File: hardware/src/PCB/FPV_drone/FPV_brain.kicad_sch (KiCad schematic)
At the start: 35 parts, among them IC2 STM32H743VIT6, IC3 USBLC6-2SC6, J1 TYPE-C-31-M-12, J3 Flash-pads, Y1 ABM3B-8.000MHZ-10-D1G-T

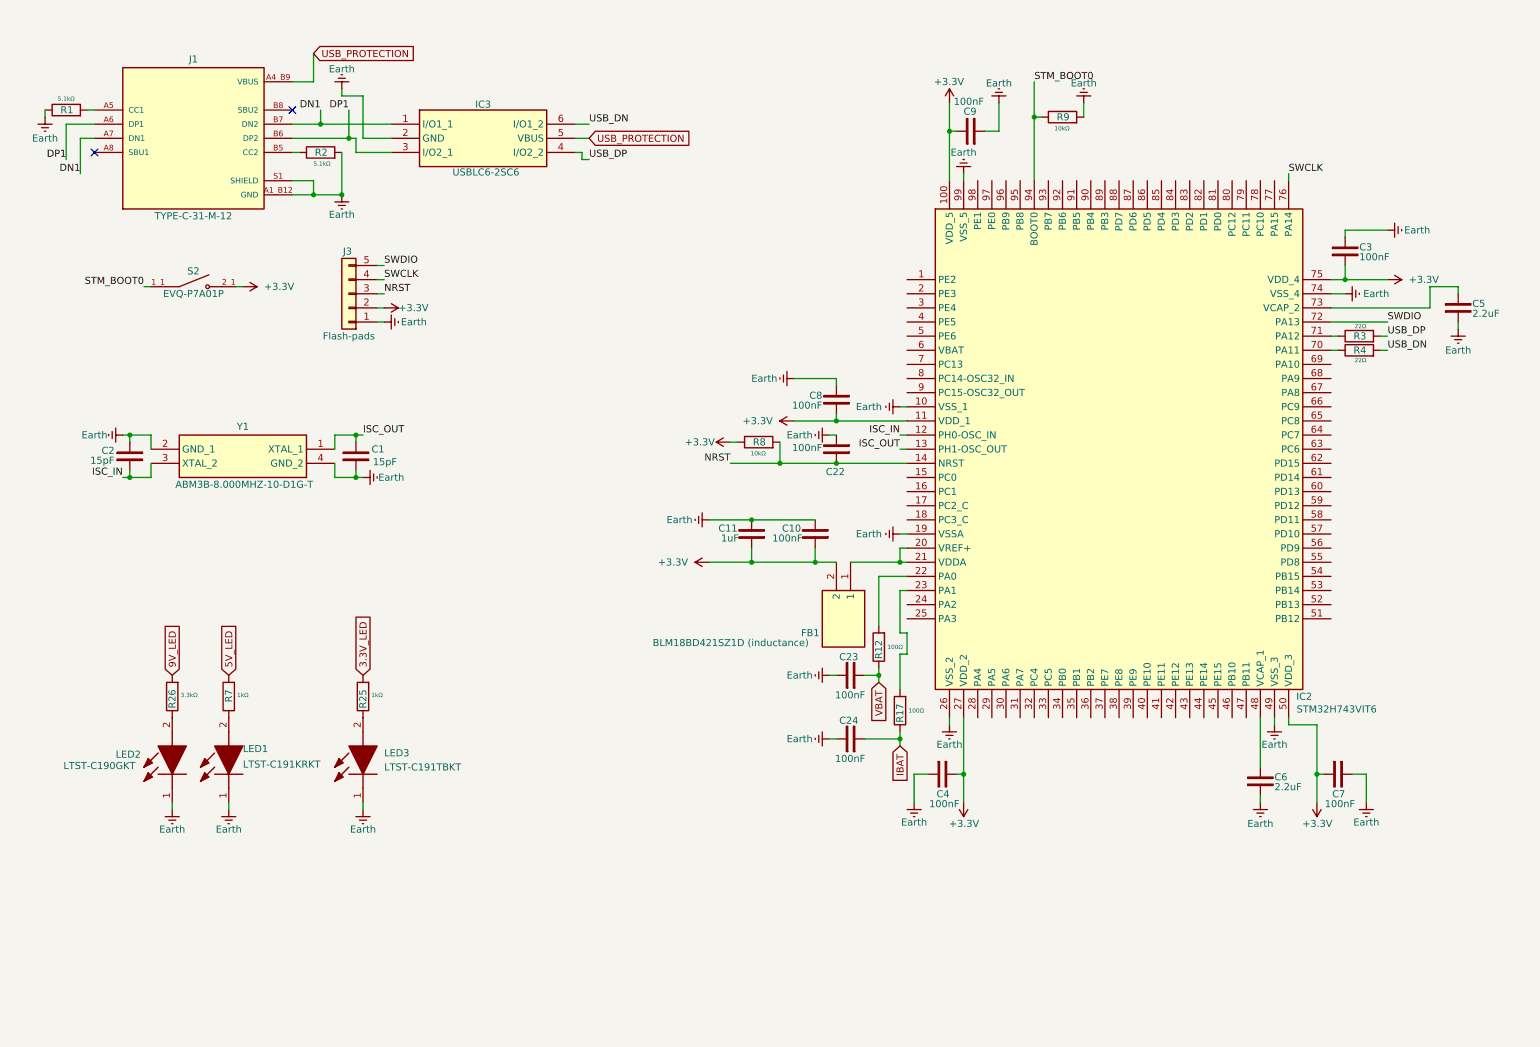
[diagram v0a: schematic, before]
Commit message: Update: schem drone
power functions almost finish... i wish
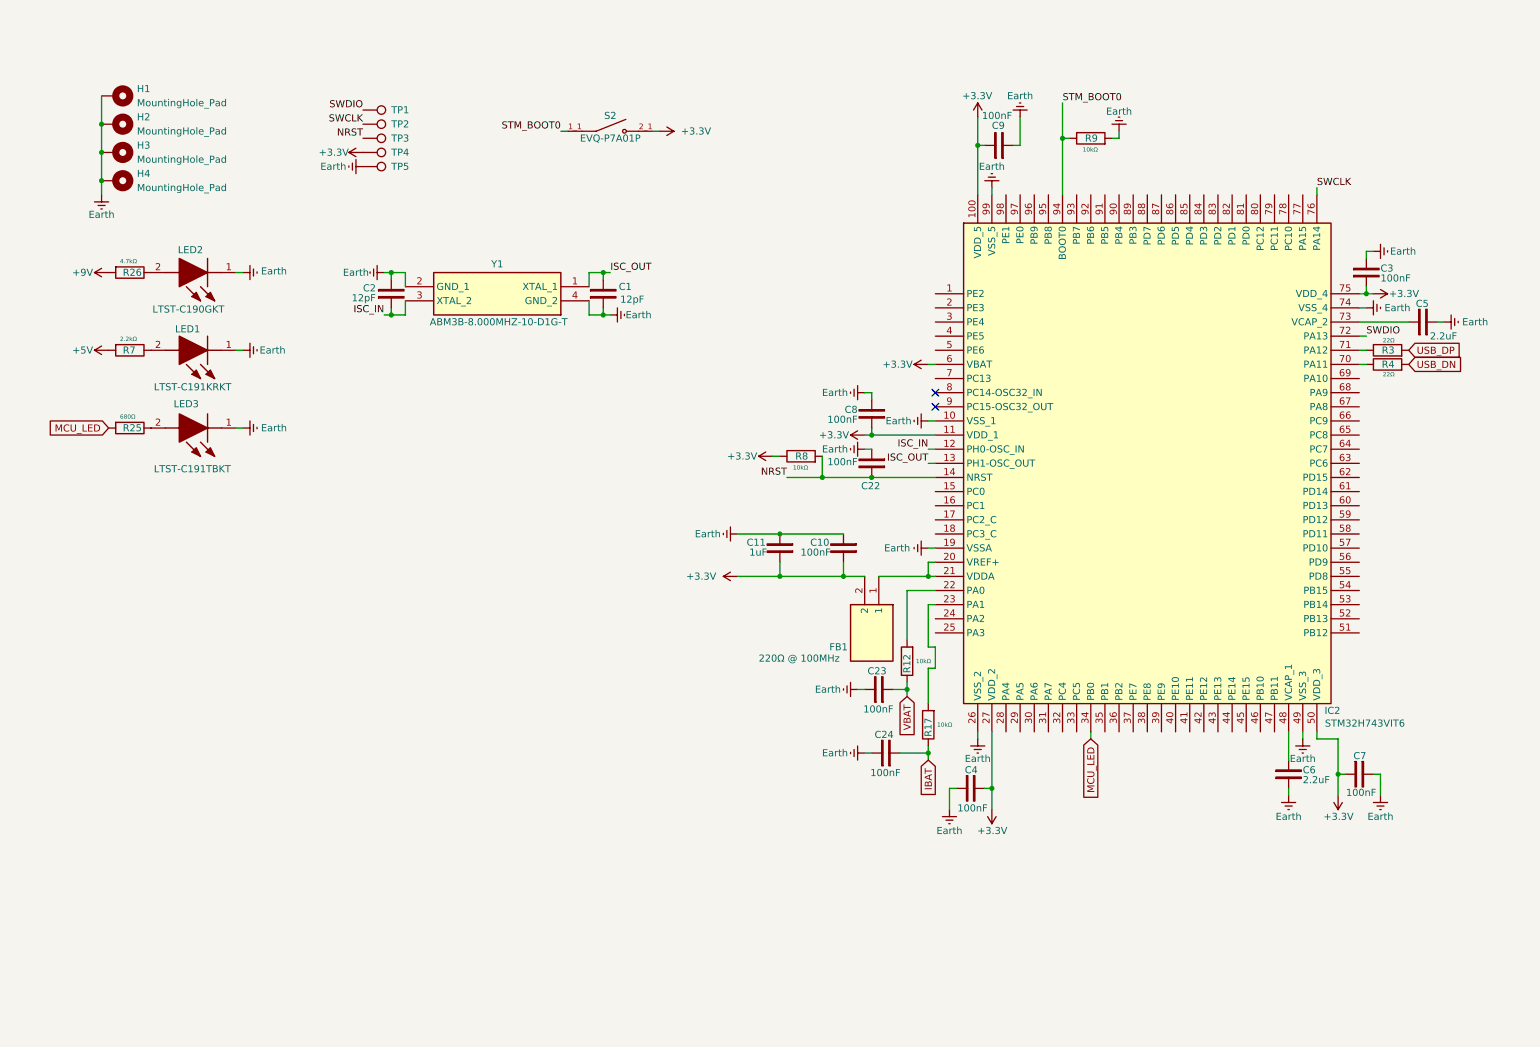
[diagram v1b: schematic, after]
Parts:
- removed IC3: USBLC6-2SC6, SOT95P280X145-6N, symbol lib:USBLC6-2SC6
- removed J1: TYPE-C-31-M-12, TYPE-C-31-M-12:HRO_TYPE-C-31-M-12, symbol lib:TYPE-C-31-M-12
- removed J3: Flash-pads, symbol Connector_Generic:Conn_01x05
- removed R1, R2: 5.1kΩ, symbol Device:R
- added H1, H2, H3, H4: MountingHole_Pad, symbol Mechanical:MountingHole_Pad
- added TP1, TP2, TP3, TP4, TP5: TestPoint, symbol Connector:TestPoint
- C1, C2: value 15pF -> 12pF
- FB1: value BLM18BD421SZ1D (inductance) -> 220Ω @ 100MHz
- R12, R17: value 100Ω -> 10kΩ
- R25: value 1kΩ -> 680Ω
- R26: value 3.3kΩ -> 4.7kΩ
- R7: value 1kΩ -> 2.2kΩ
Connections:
- net 3.3V_LED is gone; now on net MCU_LED: R25.2
- net +3.3V: now also IC2.6 (VBAT), TP4.1
- net Earth: now also H1.1, H2.1, H3.1, H4.1, TP5.1
- net NRST: now also TP3.1
- net SWCLK: now also TP2.1
- net SWDIO: now also TP1.1
- net MCU_LED: now reaches IC2.34 (PB0)
- net 5V_LED renamed +5V
- net 9V_LED renamed +9V
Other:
- moved on the sheet: C1, C10, C11, C2, C22, C23, C24, C3, C4, C5, C6, C7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

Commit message: Update: schem almost finish
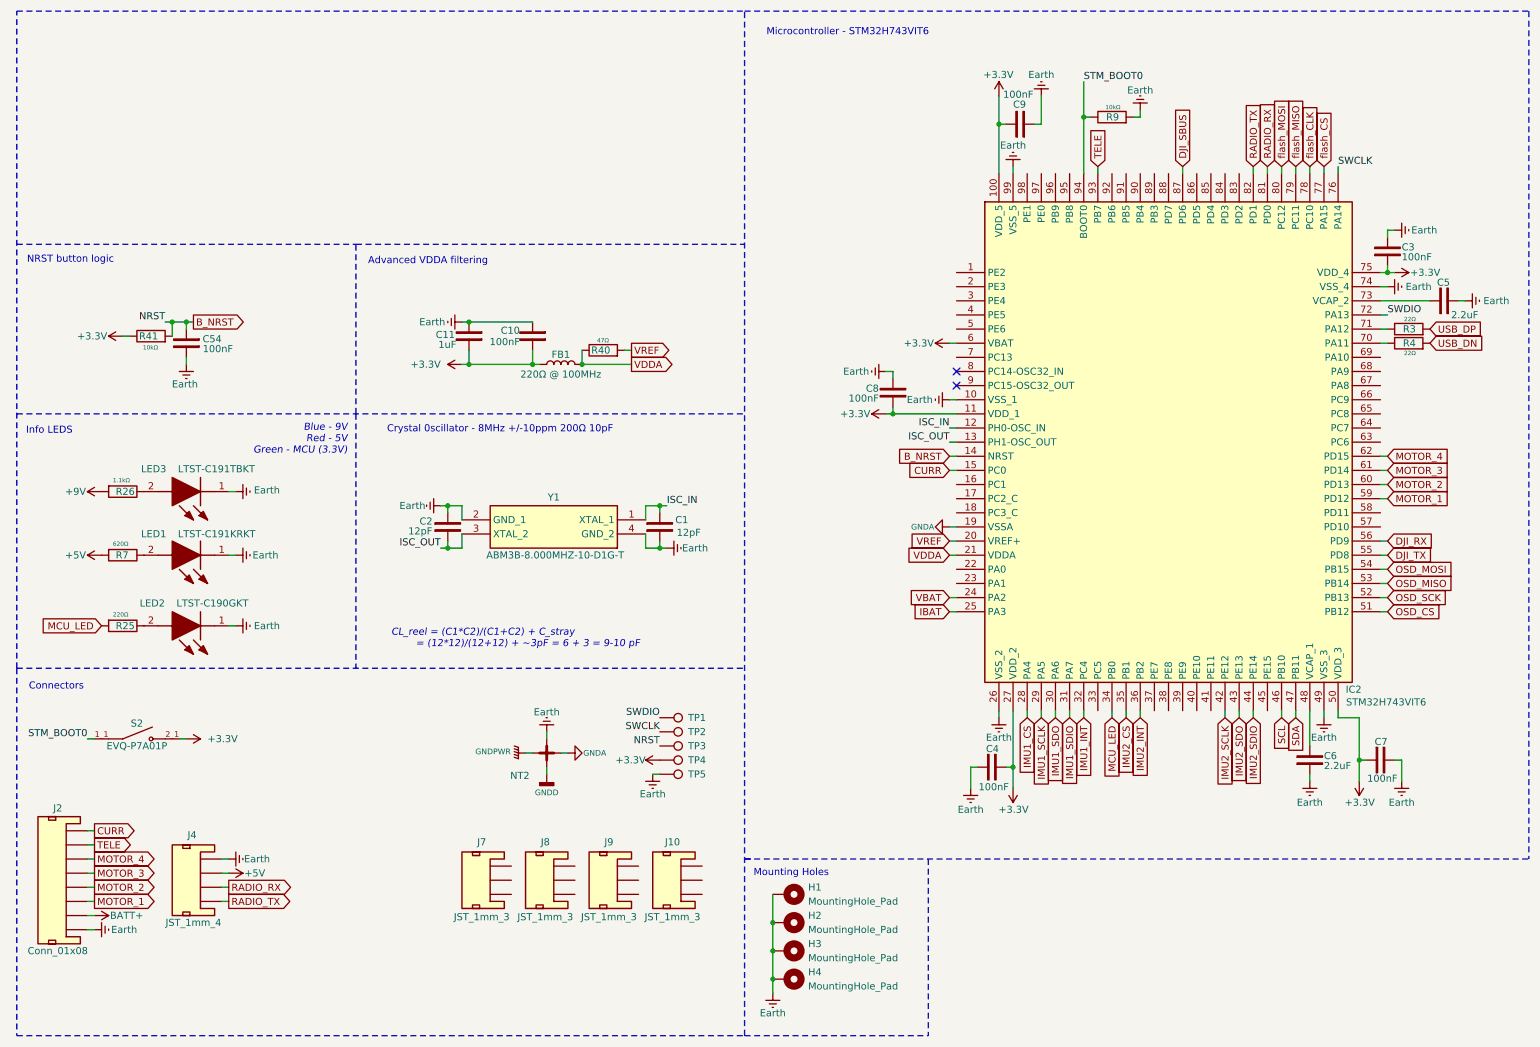
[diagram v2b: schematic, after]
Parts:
- removed C22, C23, C24: 100nF, Capacitor_THT:C_Disc_D3.0mm_W2.0mm_P2.50mm, symbol PCM_SL_Devices:Capacitor_NP
- removed FB1: 220Ω @ 100MHz, BLM18SP221SN1B, symbol lib:BLM18BD421SZ1D
- removed R12, R17, R8: 10kΩ, symbol Device:R
- added C54: 100nF, Capacitor_THT:C_Disc_D3.0mm_W2.0mm_P2.50mm, symbol PCM_SL_Devices:Capacitor_NP
- added FB1: 220Ω @ 100MHz, BLM18SP221SN1B, symbol Device:L
- added J10, J7, J8, J9: JST_1mm_3, PCM_SparkFun-Connector:JST_1x03_P1.0mm_Horizontal_SMD, symbol PCM_SparkFun-Connector:Conn_01x03_JST_P1.0mm_Horizontal_SMD
- added J2: Conn_01x08, PCM_SparkFun-Connector:JST_1x08_P1.0mm_Horizontal_SMD, symbol PCM_SparkFun-Connector:Conn_01x08_JST_P1.0mm_Horizontal_SMD
- added J4: JST_1mm_4, PCM_SparkFun-Connector:JST_1x04_P1.0mm_Horizontal_SMD, symbol PCM_SparkFun-Connector:Conn_01x04_JST_P1.0mm_Horizontal_SMD
- added NT2: NetTie_4_Cross, symbol Device:NetTie_4_Cross
- added R40: 47Ω, symbol Device:R
- added R41: 10kΩ, symbol Device:R
- R25: value 680Ω -> 220Ω
- R26: value 4.7kΩ -> 1.1kΩ
- R7: value 2.2kΩ -> 620Ω
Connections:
- net +3.3V: now also FB1.1, R41.1
- net +5V: now also J4.3
- net Earth: now also C54.2, J2.1, J4.4, NT2.3; no longer IC2.19 (VSSA)
- net IBAT: now also IC2.25 (PA3)
- net ISC_IN: now also C1.2, Y1.1 (XTAL_1); no longer C2.1, Y1.3 (XTAL_2)
- net ISC_OUT: now also C2.1, Y1.3 (XTAL_2); no longer C1.2, Y1.1 (XTAL_1)
- net VBAT: now also IC2.24 (PA2)
- net at LED3.2 (A): now also R26.1; no longer R25.1
- net at LED2.2 (A): now also R25.1; no longer R26.1
- net CURR: now reaches IC2.15 (PC0)
- net CURR: now also J2.8
- net VDDA: now reaches IC2.21 (VDDA)
- net VDDA: now also FB1.2, R40.1; no longer IC2.20 (VREF+)
- net IMU1_CS: now reaches IC2.28 (PA4)
- net IMU1_SCLK: now reaches IC2.29 (PA5)
- net IMU1_SDO: now reaches IC2.30 (PA6)
- net IMU1_SDIO: now reaches IC2.31 (PA7)
- net IMU1_INT: now reaches IC2.32 (PC4)
- net IMU2_CS: now reaches IC2.35 (PB1)
- net IMU2_INT: now reaches IC2.36 (PB2)
- net IMU2_SCLK: now reaches IC2.42 (PE12)
- net IMU2_SDO: now reaches IC2.43 (PE13)
- net IMU2_SDIO: now reaches IC2.44 (PE14)
- net SCL: now reaches IC2.46 (PB10)
- net SDA: now reaches IC2.47 (PB11)
- net OSD_CS: now reaches IC2.51 (PB12)
- net OSD_SCK: now reaches IC2.52 (PB13)
- net OSD_MISO: now reaches IC2.53 (PB14)
- net OSD_MOSI: now reaches IC2.54 (PB15)
- net DJI_TX: now reaches IC2.55 (PD8)
- net DJI_RX: now reaches IC2.56 (PD9)
- net MOTOR_1: now reaches IC2.59 (PD12)
- net MOTOR_1: now also J2.3
- net MOTOR_2: now reaches IC2.60 (PD13)
- net MOTOR_2: now also J2.4
- net MOTOR_3: now reaches IC2.61 (PD14)
- net MOTOR_3: now also J2.5
- net MOTOR_4: now reaches IC2.62 (PD15)
- net MOTOR_4: now also J2.6
- net flash_CS: now reaches IC2.77 (PA15)
- net flash_CLK: now reaches IC2.78 (PC10)
- net flash_MISO: now reaches IC2.79 (PC11)
- net flash_MOSI: now reaches IC2.80 (PC12)
- net RADIO_RX: now reaches IC2.81 (PD0)
- net RADIO_RX: now also J4.2
- net RADIO_TX: now reaches IC2.82 (PD1)
- net RADIO_TX: now also J4.1
- net DJI_SBUS: now reaches IC2.87 (PD6)
- net TELE: now reaches IC2.93 (PB7)
- net TELE: now also J2.7
- net NRST renamed B_NRST
- net B_NRST: now also C54.1, R41.2
- new net BATT+: J2.2
- new net GNDA: IC2.19 (VSSA), NT2.2
- new net GNDD: NT2.4
- new net GNDPWR: NT2.1
- new net VREF: IC2.20 (VREF+), R40.2
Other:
- note added: "Advanced VDDA filtering"
- note added: "Blue - 9V Red - 5V Green - MCU (3.3V)"
- note added: "CL_reel = (C1*C2)/(C1+C2) + C_stray = (12*12)/(12+12) + ~3pF = 6 + 3 = 9-10 pF"
- note added: "Connectors"
- note added: "Crystal 0scillator - 8MHz +/-10ppm 200Ω 10pF"
- note added: "Info LEDS"
- note added: "Microcontroller - STM32H743VIT6"
- note added: "Mounting Holes"
- note added: "NRST button logic"
- moved on the sheet: C1, C10, C11, C2, C3, C4, C5, C6, C7, C8, C9, H1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
